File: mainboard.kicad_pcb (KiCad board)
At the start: 4 copper layers, 25 x 25 mm, 135 parts, among them J1 PAD, J10 PAD, J11 Conn_02x05_Odd_Even_MountingP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, J12 Conn_02x05_Odd_Even_MountingP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, J13 PAD, J14 PAD, J15 PAD, J16 PAD, J2 PAD, J3 PAD, J4 PAD, J5 PAD, J6 PAD, J7 PAD, J8 PAD, J9 PAD, Q1 CSD75208W1015, Q2 CSD75208W1015, Q3 CSD75208W1015, Q4 2N7002, U1 SX1261, U10 TPS61099, U11 TMUX1209, U12 TMUX1209, U13 OPA333xxDCK, U2 PE4259, U3 REF3020, U4 STM32L072CBYx, U5 TMUX1209, U6 LPV542, U7 LMT70, U8 TMUX1209, U9 LPV542, Y1 32MHz

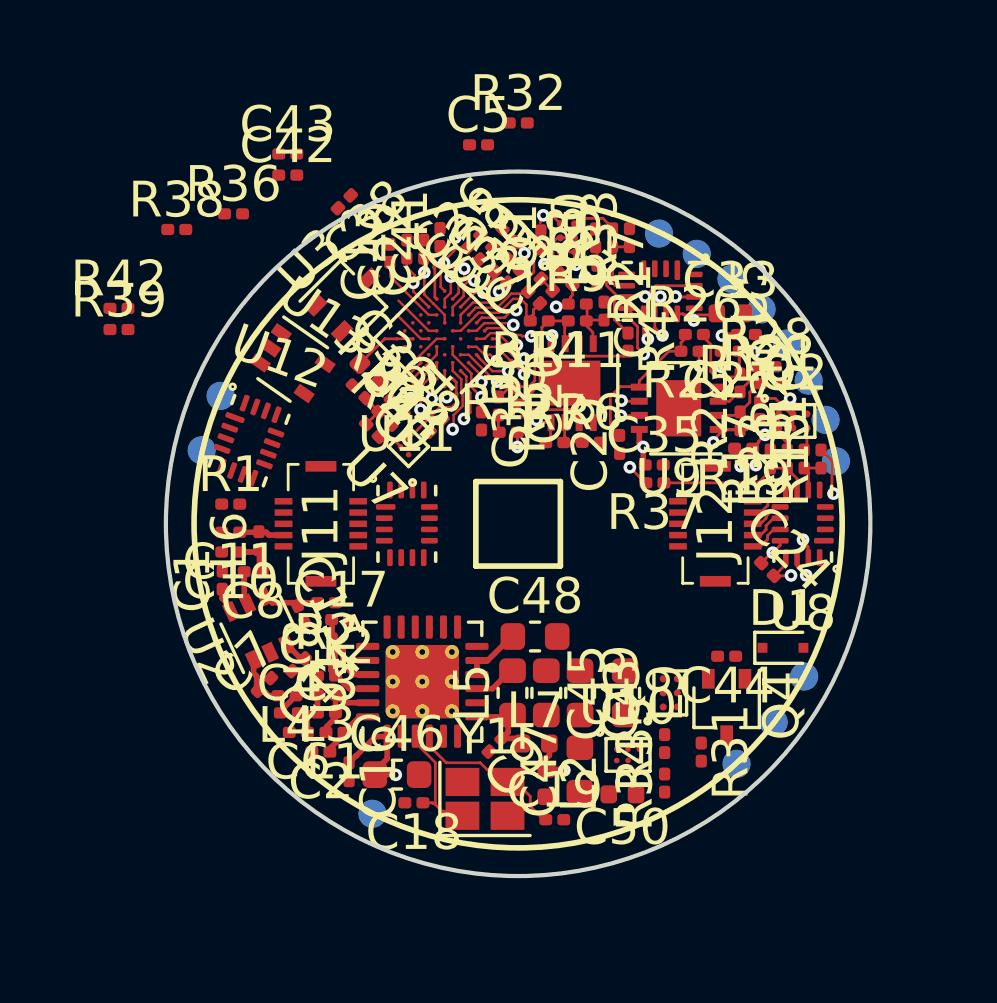
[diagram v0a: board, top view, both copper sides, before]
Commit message: finished routing
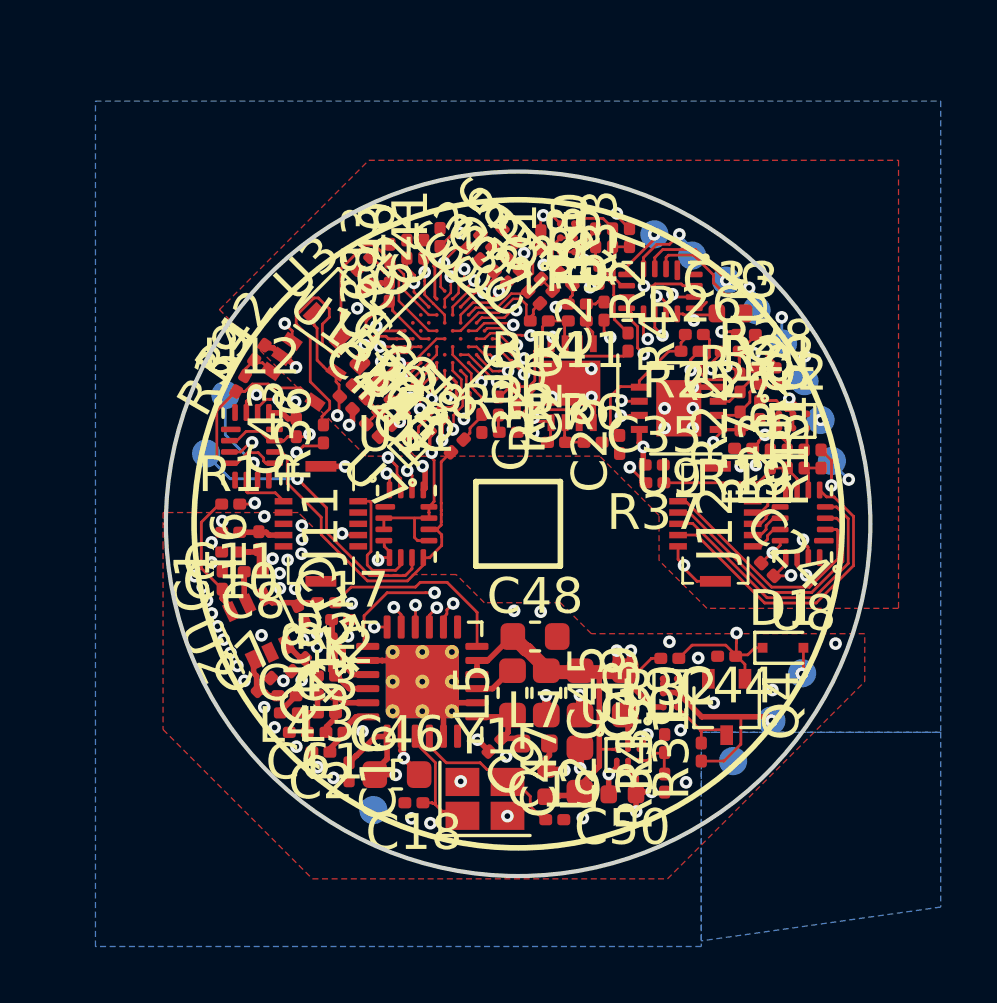
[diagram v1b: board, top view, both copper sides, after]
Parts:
- moved R32 19.7 mm to (115.4, 84.8), turned to 180 degrees
- moved R38 12.6 mm to (107.8, 77.2), turned to 45 degrees
- moved C43 9.72 mm to (102.1, 76.6), turned to 90 degrees
- moved R36 8.44 mm to (103.1, 76.8), turned to 90 degrees
- moved C42 8.34 mm to (103.9, 75.7), turned to 315 degrees
- moved C5 5.85 mm to (104.5, 70.8), turned to 225 degrees
- moved R42 5.22 mm to (100.8, 73.9), turned to 55 degrees
- moved R39 4.72 mm to (100.1, 75.0), turned to 60 degrees
- moved C38 3.58 mm to (105.4, 71.8), turned to 90 degrees
- moved U13 0.49 mm to (102.4, 74.6)
- moved U3 0.29 mm to (103.9, 72.3)
- moved U12 0.22 mm to (100.6, 77.2), turned to 0 degrees
- moved J7 0.20 mm to (117.4, 71.4)
- moved J13 0.20 mm to (98.9, 77.5)
- moved J5 0.18 mm to (118.5, 72.4)
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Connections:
- C13 pad 2: GNDA -> GNDD
- C21 pad 1: GNDA -> GNDD
- C29 pad 1: GNDA -> GNDD
- C42 pad 1: VCC -> +5VA
- C43 pad 1: VCC -> +5VA
- J1 pad 1: REFFET2_D1 -> ISFET2_D2
- J10 pad 1: ISFET2_D1 -> REFFET2_D4
- J12 pad 10: REFFET1_D4 -> REFFET1_D1
- J12 pad 4: REFFET1_D1 -> REFFET1_D4
- J12 pad 6: REFFET1_D2 -> REFFET1_D3
- J12 pad 8: REFFET1_D3 -> REFFET1_D2
- J2 pad 1: REFFET2_D2 -> ISFET2_D3
- J3 pad 1: REFFET2_D3 -> ISFET2_D4
- J4 pad 1: REFFET2_D4 -> ISFET2_D1
- J5 pad 1: ISFET2_D4 -> REFFET2_D1
- J7 pad 1: ISFET2_D3 -> REFFET2_D2
- J9 pad 1: ISFET2_D2 -> REFFET2_D3
- R12 pad 2: DAC_OUT2 -> DAC_OUT1
- R19 pad 2: ADC_IN3 -> ADC_IN6
- R21 pad 2: GNDA -> GNDD
- R27 pad 2: ADC_IN7 -> ADC_IN3
- R28 pad 2: DAC_OUT2 -> DAC_OUT1
- R33 pad 2: ADC_IN9 -> ADC_IN12
- R37 pad 2: ADC_IN6 -> ADC_IN7
- R38 pad 2: ADC_IN12 -> ADC_IN9
- R6 pad 2: GNDA -> GNDD
- U13 pad 1: DAC_OUT1 -> DAC_OUT2
- U3 pad 3: GNDA -> GNDD
- U4 pad A3: RF_CLK -> RF_SCK
- U4 pad A6: Net-(U4-PadA6) -> MUX4IN0
- U4 pad B5: Net-(U4-PadB5) -> MUX4IN1
- U4 pad B7: Net-(U4-PadB7) -> ANT_SW
- U4 pad C1: Net-(U4-PadC1) -> MUX3IN1
- U4 pad D1: Net-(U4-PadD1) -> RF_RST
- U4 pad D2: Net-(U4-PadD2) -> RF_BUSY
- U4 pad E1: Net-(U4-PadE1) -> AFE_EN
- U4 pad E2: Net-(U4-PadE2) -> MUX3EN
- U4 pad F1: Net-(U4-PadF1) -> TAG_EN
- U4 pad F2: Net-(U4-PadF2) -> MUX1IN0
- U4 pad F3: Net-(U4-PadF3) -> MUX3IN0
- U4 pad G1: Net-(U4-PadG1) -> MUX1IN1
- U5 pad 14: MUX1IN1 -> MUX2IN1
- U5 pad 15: MUX1IN0 -> MUX2IN0
- U7 pad A1: GNDA -> GNDD
- U8 pad 14: MUX2IN1 -> MUX1IN1
- U8 pad 15: MUX2IN0 -> MUX1IN0
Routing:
- net VCC: track 8.77 -> 40.5 mm, vias 3 -> 6
- net GNDD: track 3.79 -> 30.6 mm, vias 2 -> 78
- net DAC_OUT1: track 1.74 -> 24.0 mm, vias 1 -> 3
- net TAG_EN: track 0.00 -> 21.2 mm, vias 0 -> 2
- net ADC_IN2: track 4.36 -> 24.4 mm
- net AFE_EN: track 0.00 -> 18.4 mm, vias 0 -> 2
- net +5VA: track 4.83 -> 23.0 mm, vias 4 -> 9
- net MUX1IN1: track 0.71 -> 18.0 mm, vias 1 -> 2
- net MUX1IN0: track 1.90 -> 17.8 mm, vias 1 -> 2
- net ADC_IN0: track 3.28 -> 18.0 mm
- net ADC_IN6: track 2.63 -> 16.7 mm
- net ELEC_SNS2: track 0.00 -> 13.5 mm
- net RF_CS: track 0.79 -> 13.6 mm, vias 1 -> 2
- net RF_SCK: track 0.00 -> 12.2 mm, vias 0 -> 2
- net ANT_SW: track 0.00 -> 11.5 mm, vias 0 -> 2
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- added copper zone on In1.Cu, net +5VA
- added copper zone on B.Cu, net GNDD
- added copper zone on F.Cu, net GNDD
- added copper zone on In1.Cu, net VCC
